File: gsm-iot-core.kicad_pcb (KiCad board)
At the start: 2 copper layers, 25.4 x 64.8 mm, 92 parts, among them J1 MICRO_SD_HINGE - Micro SD soc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, P1 CONN_01X17, P2 CONN_01X17, P3 Chip anten, Q1 2SC1815, Q2 2SC1815, SW1 SW_PUSH, SW2 SW_PUSH, U1 MP2365DN, U2 LP2985-50DBVR, U3 STM32F405RGTx, U4 MMA7660, U5 SIM800C, U6 SIM HOLD - PPSS-6P, X1 CRYSTAL-24M, Y1 32.768MHz

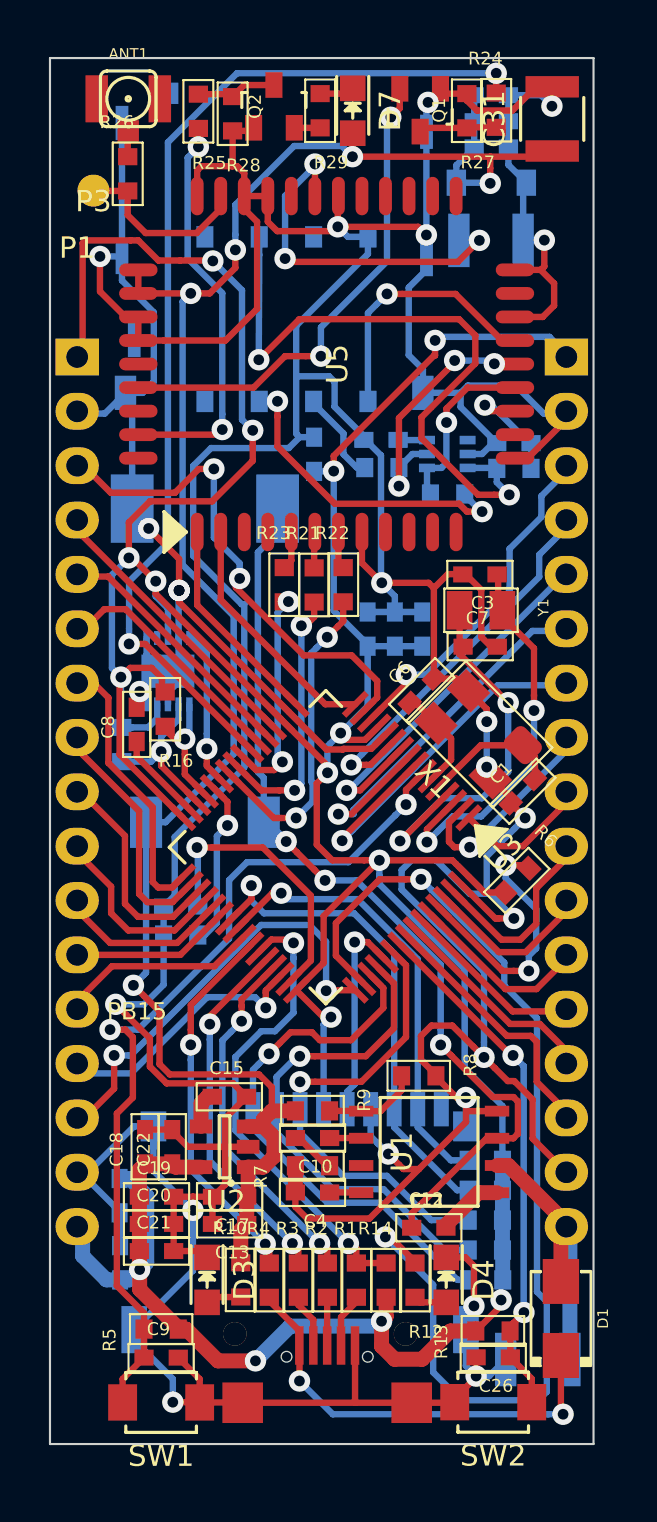
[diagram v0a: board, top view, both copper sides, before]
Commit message: Final pcb
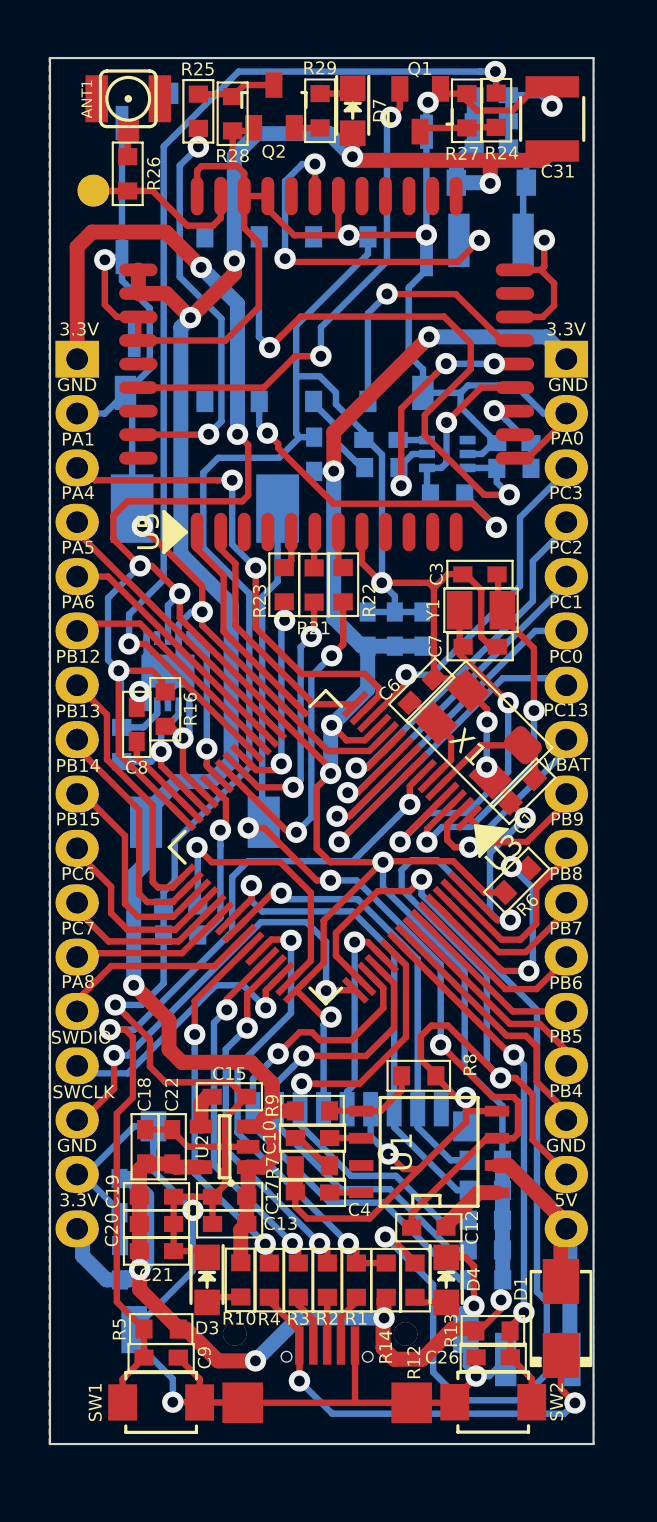
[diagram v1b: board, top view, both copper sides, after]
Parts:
- moved P1 0.10 mm to (149.6, 78.7)
- moved P2 0.10 mm to (172.5, 78.7)
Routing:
- net +3V3: track 196.9 -> 199.4 mm
- net Net-(D5-Pad3): track 30.9 -> 29.0 mm
- net VDD: track 91.1 -> 92.8 mm
- net Net-(R19-Pad1): track 15.0 -> 16.5 mm
- net SIM800C_DATA: track 5.65 -> 4.50 mm
- net SIM800C_RI: track 15.1 -> 16.0 mm
- net GND: track 375.1 -> 374.2 mm, vias 23 -> 22
- net PA15_LED: track 49.7 -> 49.0 mm
- net GSM_ANT: track 8.50 -> 7.79 mm
- net Net-(R6-Pad2): track 12.3 -> 11.7 mm
- net PA6: track 11.2 -> 10.7 mm
- net PA10_ID: track 22.2 -> 21.7 mm
- added copper zone on B.Cu, net GND
- added copper zone on F.Cu, net GND
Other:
- board text added: "3.3V"
- board text added: "5V"
- board text added: "GND"
- board text added: "PA0"
- board text added: "PA1"
- board text added: "PA4"
- board text added: "PA5"
- board text added: "PA6"
- board text added: "PA8"
- board text added: "PB12"
- board text added: "PB13"
- board text added: "PB14"
- board text added: "PB4"
- board text added: "PB5"
- board text added: "PB6"
- board text added: "PB7"
- board text added: "PB8"
- board text added: "PB9"
- board text added: "PC0"
- board text added: "PC1"
- board text added: "PC13"
- board text added: "PC2"
- board text added: "PC3"
- board text added: "PC6"
- board text added: "PC7"
- board text added: "SWCLK"
- board text added: "SWDIO"
- board text added: "VBAT"
